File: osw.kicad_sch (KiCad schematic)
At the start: 67 parts, among them J1 Conn_01x02, Q1 2N7002, SW1 SW_Push, SW2 SW_Push, SW3 SPST_EVQ-P7J01P, U1 DS3231MZ, U10 XC6209, U11 MCP73831T-2ACI_OT, U13 XC6209, U2 BMA400, U3 PSRAM64H, U4 GC9A01_IPS_display, U5 USB-OTG, U6 CH340E, U7 ttgo-32-micro, U8 Quectel_L96, U9 TPS2115A

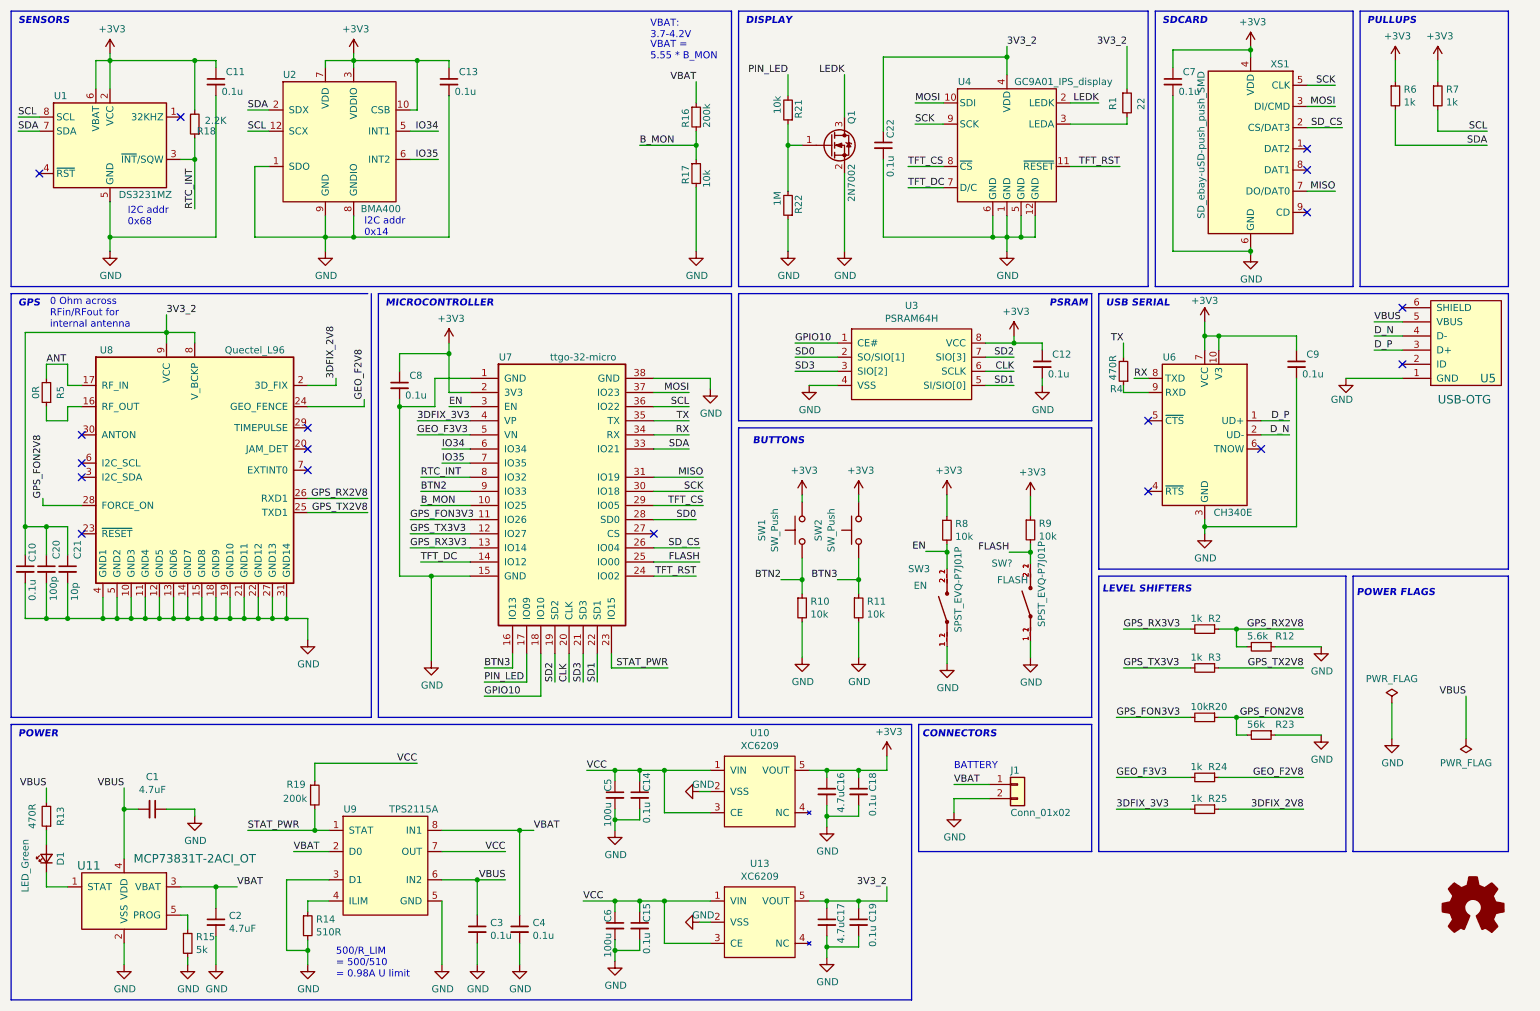
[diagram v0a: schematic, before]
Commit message: Updates to the board and schematic.
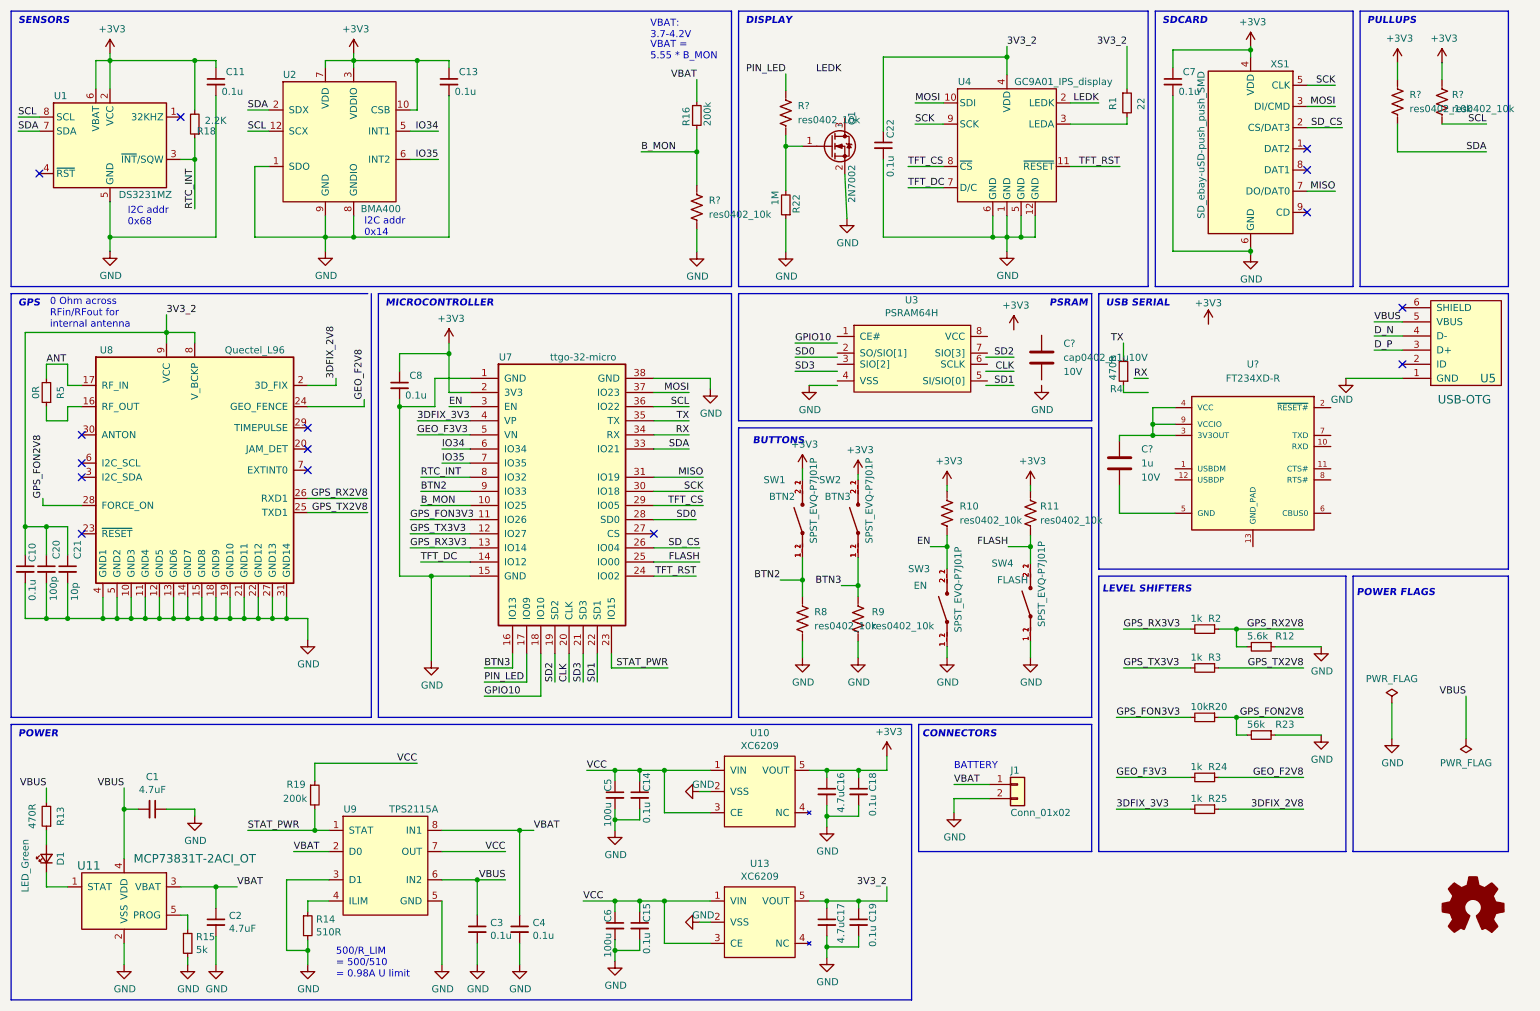
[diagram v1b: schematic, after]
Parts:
- removed C12, C9: 0.1u, Capacitor_SMD:C_0603_1608Metric, symbol Device:C_Small
- removed R10, R11, R17, R21, R8, R9: 10k, Resistor_SMD:R_0603_1608Metric, symbol Device:R_Small
- removed R6, R7: 1k, Resistor_SMD:R_0603_1608Metric, symbol Device:R_Small
- removed SW1, SW2: SW_Push, open-Smartwatch:button_side_smd, symbol Switch:SW_Push
- removed U6: CH340E, open-Smartwatch:MSOP-10_3x3mm_P0.5mm, symbol open-Smartwatch:CH340E
- added C?: 1u, open-Smartwatch:C_0402_1005Metric_osw, symbol open-Smartwatch:cap0402_p1u10V
- added C?: cap0402_p1u10V, open-Smartwatch:C_0402_1005Metric_osw, symbol open-Smartwatch:cap0402_p1u10V
- added R10, R11, R8, R9, R? (x4): res0402_10k, open-Smartwatch:R_0402_1005Metric_osw, symbol open-Smartwatch:res0402_10k
- added SW1, SW2: SPST_EVQ-P7J01P, open-Smartwatch:SW_EVQ-P7J01P, symbol open-Smartwatch:SPST_EVQ-P7J01P
- added U?: FT234XD-R, open-Smartwatch:SON45P300X300X80-13N, symbol open-Smartwatch:FT234XD-R
- gave numbers to parts that had none: 1
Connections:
- net +3V3: now also R10.1, R11.1, R?.1, R?.1, SW1.2_1, SW1.2_2, SW2.2_1, SW2.2_2; no longer U3.8 (VCC)
- net BTN2: now also R8.1, SW1.1_1, SW1.1_2
- net BTN3: now also R9.1, SW2.1_1, SW2.1_2
- net B_MON: now also R?.1
- net CLK: no longer U3.6 (SCLK)
- net EN: now also SW3.2_1, SW3.2_2, R10.2
- net FLASH: now also R11.2
- net GND: now also R8.2, R9.2, R?.2; no longer U3.4 (VSS)
- net GPIO10: no longer U3.1 (CE#)
- net LEDK: no longer Q1.3 (D)
- net PIN_LED: now also R?.1
- net SCL: now also R?.2
- net SD0: no longer U3.2 (SO/SIO[1])
- net SD1: no longer U3.5 (SI/SIO[0])
- net SD2: no longer U3.7 (SIO[3])
- net SD3: no longer U3.3 (SIO[2])
- net SDA: now also R?.2
- net at Q1.1 (G), R22.2: now also R?.2
- new net: C?.1, U?.3 (3V3OUT), U?.4 (VCC), U?.9 (VCCIO)
- new net: C?.2, U?.5 (GND)
- no-connect marks 18 -> 15
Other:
- moved on the sheet: U3
